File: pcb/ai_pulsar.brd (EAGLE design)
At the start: 66 x 66 mm, 85 parts, among them IC1 DS1307SO8-TIGHT, J1 JST-3P-MALE, J2 JST-2P-MALE, Q1 BSS138, U1 MIC5219-3.3, U2 FT231X-Q

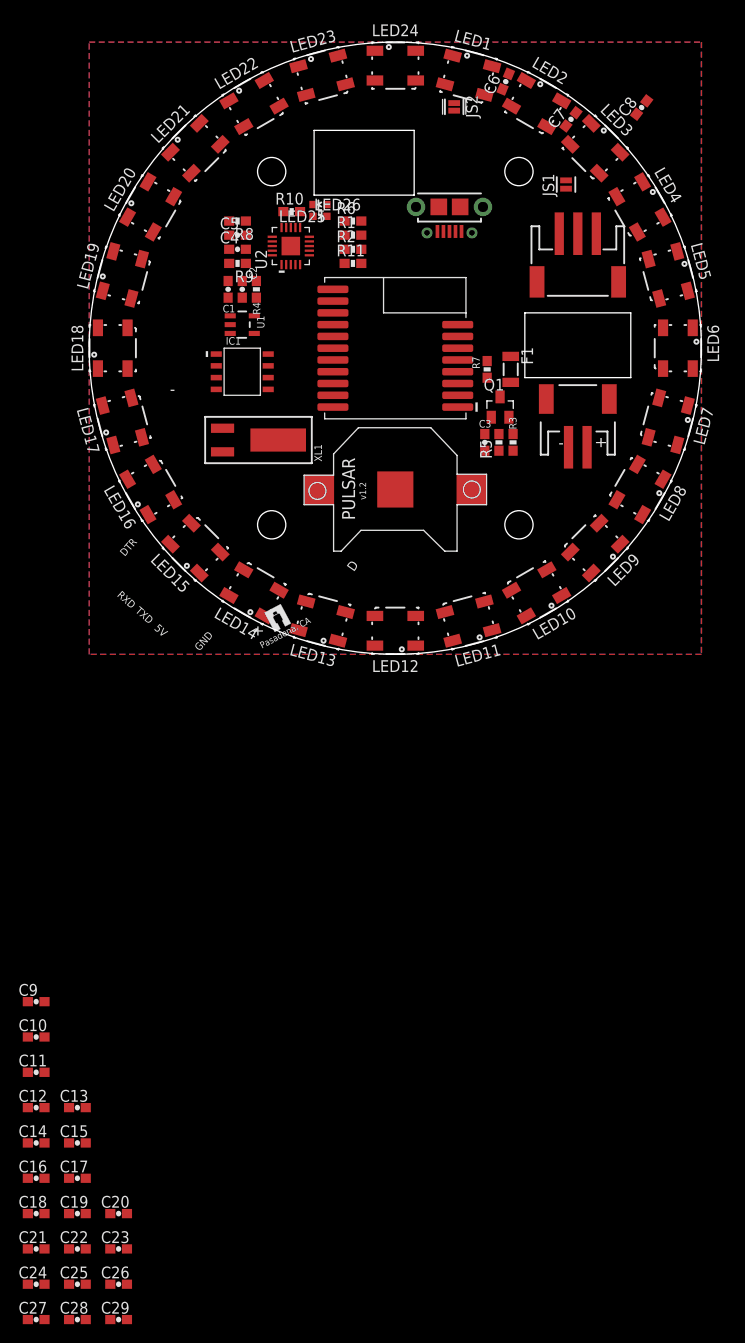
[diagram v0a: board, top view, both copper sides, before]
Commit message: routing under way
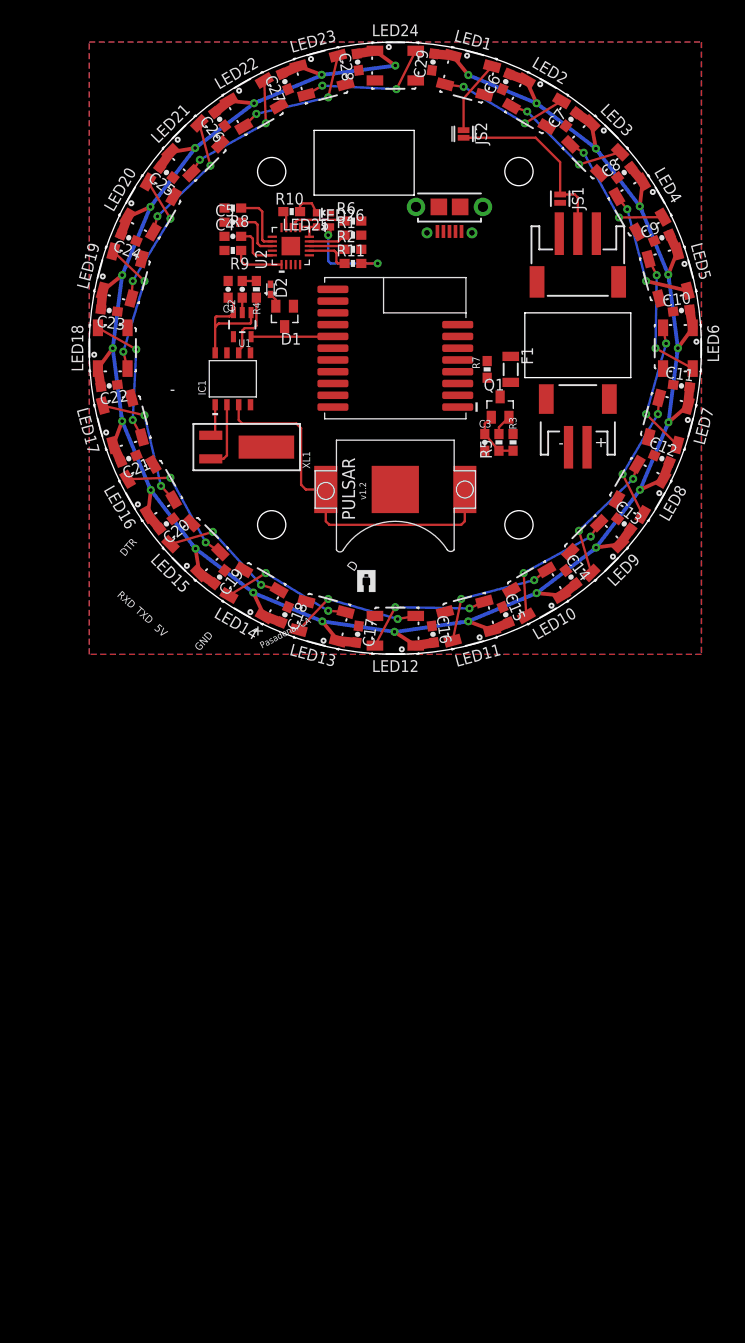
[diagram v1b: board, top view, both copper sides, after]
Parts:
- added D1: DIODE-SCHOTTKY-DUAL, Ai_DiscreteSemis:SOT-23
- added D2: (no value), Ai_DiscreteSemis:SOD-523
- 3V-BATT: device Ai_Connectors:CR1220-SMD -> Ai_Connectors:CR1025-SMD
- moved C29 139.8 mm to (37.1, 63.9), turned to 82.5 degrees
- moved C28 139.0 mm to (29.0, 63.9), turned to 97.5 degrees
- moved C27 136.2 mm to (21.1, 61.8), turned to 112.5 degrees
- moved C26 126.1 mm to (14.1, 57.7), turned to 127.5 degrees
- moved C25 120.3 mm to (8.33, 52.0), turned to 142.5 degrees
- moved C24 113.3 mm to (4.27, 44.9), turned to 157.5 degrees
- moved C9 106.5 mm to (61.8, 44.9), turned to 22.5 degrees
- moved C10 104.8 mm to (63.9, 37.1), turned to 7.5 degrees
- moved C11 101.6 mm to (63.9, 29.0), turned to 352.5 degrees
- moved C23 101.2 mm to (2.16, 37.1), turned to 172.5 degrees
- moved C12 97.2 mm to (61.8, 21.1), turned to 337.5 degrees
- moved C22 93.2 mm to (2.16, 29.0), turned to 187.5 degrees
- moved C13 86.3 mm to (57.7, 14.1), turned to 322.5 degrees
- moved C21 85.8 mm to (4.27, 21.1), turned to 202.5 degrees
- moved C14 84.0 mm to (52.0, 8.33), turned to 307.5 degrees
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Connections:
- new net +: D2.A, J2.1
- new net DI-1: LED6.2, LED7.4
- new net DI-2: LED18.2, LED19.4
- new net N$13: LED12.2, LED13.4
- new net N$16: LED2.2, LED3.4
- new net N$18: LED3.2, LED4.4
- new net N$19: LED4.2, LED5.4
- new net N$20: LED5.2, LED6.4
- new net N$21: LED7.2, LED8.4
- new net N$22: LED8.2, LED9.4
- new net N$23: LED10.4, LED9.2
- new net N$24: LED10.2, LED11.4
- new net N$25: LED11.2, LED12.4
- new net N$26: LED13.2, LED14.4
- new net N$27: LED14.2, LED15.4
- new net N$28: LED15.2, LED16.4
- new net N$29: LED16.2, LED17.4
- new net N$32: LED17.2, LED18.4
- new net N$33: LED19.2, LED20.4
- new net N$34: LED20.2, LED21.4
- new net N$35: LED21.2, LED22.4
- new net N$36: LED22.2, LED23.4
- new net N$37: LED23.2, LED24.4
- new net VBAT: D1.2, D2.C
- new net VCC: C1.1, C10.2, C11.2, C12.2, C13.2, C14.2, C15.2, C16.2, C17.2, C18.2, C19.2, C20.2, C21.2, C22.2, C23.2, C24.2, C25.2, C26.2, C27.2, C28.2, C29.2, C6.2, C7.2, C8.2, C9.2, D1.3, IC1.8, LED1.1, LED10.1, LED11.1, LED12.1, LED13.1, LED14.1, LED15.1, LED16.1, LED17.1, LED18.1, LED19.1, LED2.1, LED20.1, LED21.1, LED22.1, LED23.1, LED24.1, LED3.1, LED4.1, LED5.1, LED6.1, LED7.1, LED8.1, LED9.1, R6.1, U1.1, U1.3, U2.12
- net 5V: now also D1.1; no longer C1.1, C6.2, C7.2, IC1.8, LED1.1, LED2.1, LED3.1, R6.1, U1.1, U1.3, U2.12
- net GND: now also C10.1, C11.1, C12.1, C13.1, C14.1, C15.1, C16.1, C17.1, C18.1, C19.1, C20.1, C21.1, C22.1, C23.1, C24.1, C25.1, C26.1, C27.1, C28.1, C29.1, C8.1, C9.1, J2.2, LED10.3, LED11.3, LED12.3, LED13.3, LED14.3, LED15.3, LED16.3, LED17.3, LED18.3, LED19.3, LED20.3, LED21.3, LED22.3, LED23.3, LED24.3, LED3.3, LED4.3, LED5.3, LED6.3, LED7.3, LED8.3, LED9.3
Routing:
- net VCC: track 0.00 -> 319.3 mm, vias 0 -> 24
- net N$1: track 0.00 -> 39.9 mm
- net D: track 0.00 -> 20.9 mm
- net 3V3: track 0.00 -> 16.3 mm
- net N$37: track 0.00 -> 14.6 mm, vias 0 -> 2
- net N$23: track 0.00 -> 14.6 mm, vias 0 -> 2
- net N$27: track 0.00 -> 14.5 mm, vias 0 -> 2
- net N$36: track 0.00 -> 14.5 mm, vias 0 -> 2
- net N$32: track 0.00 -> 14.5 mm, vias 0 -> 2
- net N$24: track 0.00 -> 14.5 mm, vias 0 -> 2
- net DI-2: track 0.00 -> 14.5 mm, vias 0 -> 2
- net N$29: track 0.00 -> 14.5 mm, vias 0 -> 2
- net N$22: track 0.00 -> 14.5 mm, vias 0 -> 2
- net N$25: track 0.00 -> 14.5 mm, vias 0 -> 2
- net N$28: track 0.00 -> 14.5 mm, vias 0 -> 2
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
